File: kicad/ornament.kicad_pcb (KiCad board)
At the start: 4 copper layers, 104.6 x 99.5 mm, 129 parts, among them J1 10118193-0001LF, J2 Conn_02x03_Odd_Even, SW1 SW_Push, U1 ATmega328P-AU, U2 MCP73831T-2ACI_OT, Y1 8Mhz

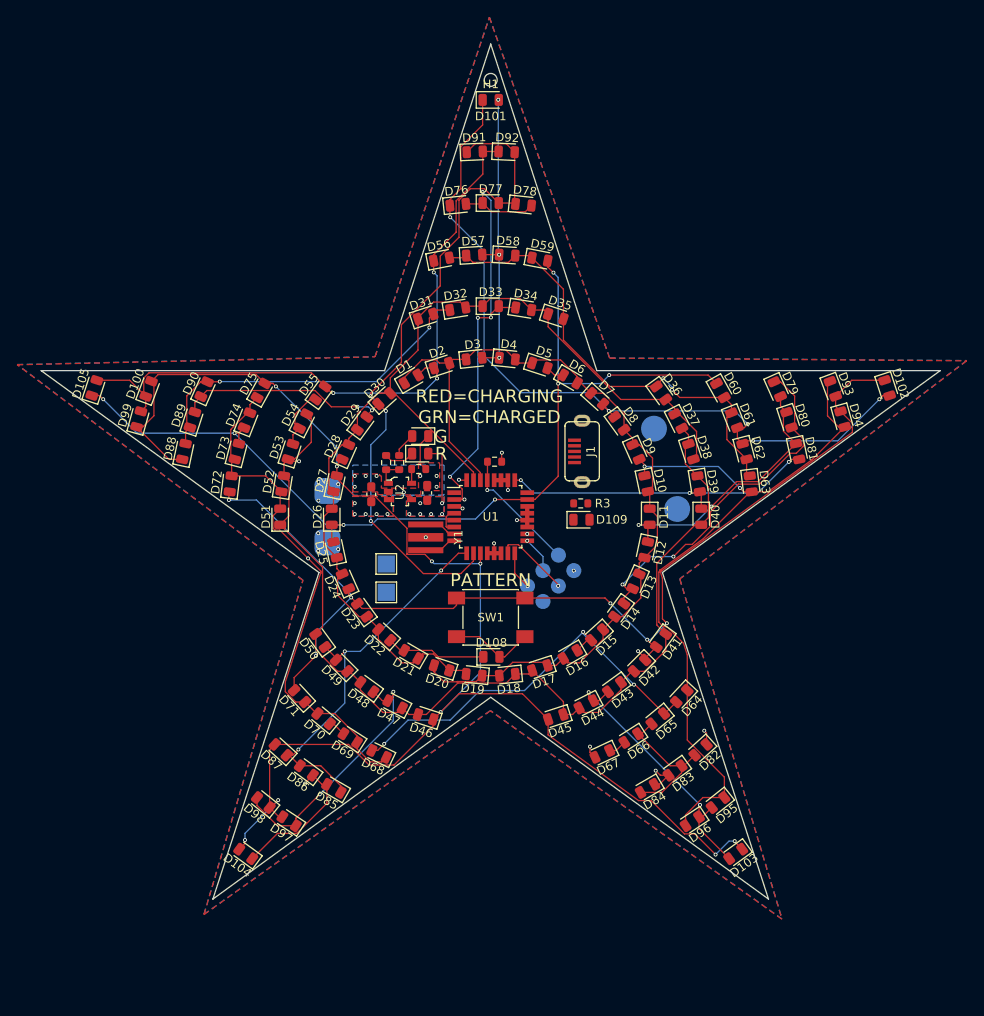
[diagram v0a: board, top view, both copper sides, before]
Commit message: 23JAN2021
90% PCB layout
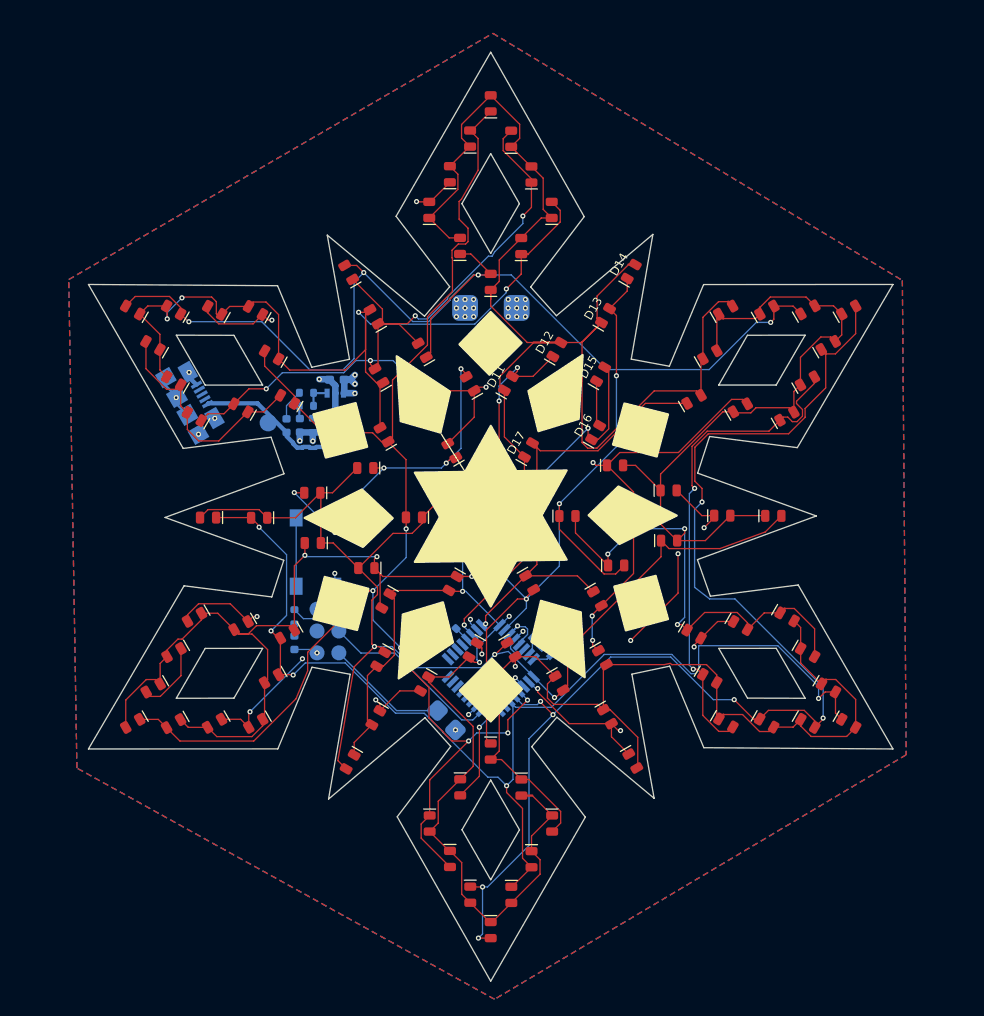
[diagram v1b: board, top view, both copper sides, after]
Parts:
- removed D106: RED, LED_SMD:LED_0805_2012Metric
- removed D107: GREEN, LED_SMD:LED_0805_2012Metric
- removed D108: D, Diode_SMD:D_0805_2012Metric
- removed D109: YELLOW, LED_SMD:LED_0805_2012Metric
- removed G***: LOGO, Joshua:Handmade_Electronics-15.2x10.2mm
- removed H1: MountingHole, Joshua:MountingHole_1.5mm
- removed TP4: USB GND TestPoint, Joshua:POGO_CONTACT_PAD_3MM
- C1, C3, R1, R2, R3, R4, R6, SW1, TP5, TP6, U1, U2, Y1: moved to B.Cu
- D103: value LED_Small -> RED; footprint LED_SMD:LED_0805_2012Metric -> Diode_SMD:D_0603_1608Metric; moved to B.Cu
- D104: value LED_Small -> GREEN; footprint LED_SMD:LED_0805_2012Metric -> Diode_SMD:D_0603_1608Metric; moved to B.Cu
- D105: value LED_Small -> YELLOW; footprint LED_SMD:LED_0805_2012Metric -> Diode_SMD:D_0603_1608Metric; moved to B.Cu
- J1: footprint Joshua:USB-B_Micro_Female_Vertical_2073-USB3140-30-0230-1 -> digikey-footprints:USB_Micro_B_Female_10118192; moved to B.Cu
- moved D57 78.6 mm to (100.0, 148.1), turned to 270 degrees
- moved D58 74.5 mm to (97.6, 144.0), turned to 270 degrees
- moved D56 74.4 mm to (102.4, 144.0), turned to 270 degrees
- moved D95 73.6 mm to (74.5, 81.2), turned to 150 degrees
- moved D93 72.5 mm to (67.9, 76.0), turned to 150 degrees
- moved D103 72.2 mm to (76.2, 89.4), turned to 270 degrees
- moved D59 70.6 mm to (95.3, 139.8), turned to 270 degrees
- moved D94 69.5 mm to (72.6, 76.0), turned to 150 degrees
- moved D23 66.5 mm to (141.7, 75.9), turned to 30 degrees
- moved D82 63.4 mm to (67.1, 100.1), turned to 180 degrees
- moved D81 63.1 mm to (73.1, 100.1), turned to 180 degrees
- moved D24 62.5 mm to (139.3, 80.1), turned to 30 degrees
- moved D22 62.1 mm to (136.9, 75.9), turned to 30 degrees
- moved D76 61.7 mm to (63.1, 115.8), turned to 210 degrees
- moved D60 60.7 mm to (92.9, 135.7), turned to 270 degrees
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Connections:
- D103 pad 1: PIN8 -> Net-(D103-Pad1)
- D103 pad 2: PIN9 -> +5V
- D104 pad 1: PIN9 -> GND
- D104 pad 2: PIN8 -> Net-(D104-Pad2)
- D105 pad 1: PIN9 -> GND
- D105 pad 2: PIN11 -> Net-(D105-Pad2)
- R1 pad 2: Net-(D106-Pad1) -> Net-(D103-Pad1)
- R2 pad 2: Net-(D107-Pad2) -> Net-(D104-Pad2)
- R3 pad 1: Net-(D109-Pad2) -> Net-(D105-Pad2)
- U1 pad 12: GND -> PIN9
- U1 pad 13: GND -> PIN10
- U1 pad 14: GND -> PIN11
- U1 pad 19: GND -> Net-(U1-Pad19)
- U1 pad 20: GND -> Net-(U1-Pad20)
- U1 pad 22: GND -> Net-(U1-Pad22)
- U1 pad 23: PIN9 -> Net-(U1-Pad23)
- U1 pad 24: PIN10 -> Net-(U1-Pad24)
- U1 pad 25: PIN11 -> Net-(U1-Pad25)
- U1 pad 26: GND -> Net-(U1-Pad26)
- U1 pad 27: GND -> Net-(U1-Pad27)
- U1 pad 28: GND -> Net-(U1-Pad28)
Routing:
- net PIN10: track 178.6 -> 315.0 mm, vias 11 -> 17
- net PIN11: track 166.3 -> 262.3 mm, vias 7 -> 9
- net PIN1: track 102.5 -> 172.7 mm, vias 0 -> 1
- net PIN8: track 265.5 -> 206.1 mm, vias 14 -> 12
- net PIN4: track 113.9 -> 173.3 mm
- net PIN9: track 198.4 -> 254.8 mm, vias 10 -> 8
- net PIN6: track 137.5 -> 193.2 mm, vias 7 -> 5
- net PIN2: track 119.3 -> 157.6 mm, vias 0 -> 4
- net PIN3: track 139.2 -> 172.4 mm
- net PIN7: track 223.5 -> 191.1 mm, vias 9 -> 11
- net SCK: track 4.23 -> 27.6 mm, vias 1 -> 0
- net +5V: track 7.35 -> 26.8 mm, vias 6 -> 3
- net PIN5: track 200.8 -> 181.7 mm, vias 9 -> 6
- net GND: track 14.7 -> 33.7 mm, vias 17 -> 23
- net MOSI: track 8.92 -> 0.00 mm, vias 1 -> 0
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- added copper zone on In1.Cu, net +VBAT
- added copper zone on In2.Cu, net GND
- removed copper zone on B.Cu, net +5V
- removed copper zone on F.Cu, net +5V
- removed copper zone on B.Cu, net +VBAT
- removed copper zone on F.Cu, net +VBAT
- removed copper zone on In2.Cu, net +VBAT
- removed copper zone on B.Cu, net GND
- removed copper zone on F.Cu, net GND
- removed copper zone on In1.Cu, net GND
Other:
- board size 104.6 x 99.5 mm -> 93.6 x 108.1 mm
- net class +VBAT: clearance 0.127 -> 0.1524; trace_width 0.127 -> 0.1524; via_dia 0.4572 -> 0.6; via_drill 0.254 -> 0.3
- net class Default: clearance 0.0889 -> 0.1524; trace_width 0.0889 -> 0.1524; via_dia 0.4572 -> 0.6; via_drill 0.254 -> 0.3
- net class GND: clearance 0.127 -> 0.1524; trace_width 0.127 -> 0.762; via_dia 0.4572 -> 0.6; via_drill 0.254 -> 0.3
- rule trace_clearance: 0.0889 -> 0.1524
- board text added: "+"
- board text added: "-"
- board text added: "1"
- board text added: "PATTERN CHANGE"
- board text removed: "G"
- board text removed: "PATTERN"
- board text removed: "R"
- board text removed: "RED=CHARGING GRN=CHARGED"
